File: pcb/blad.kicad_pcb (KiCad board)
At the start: 2 copper layers, 228.6 x 76.2 mm, 117 parts, among them J1 HRO_TYPE-C-31-M-12, J2 SWD, Q1 AO3401A, SW1 1U, SW10 1U, SW11 1U, SW12 1U, SW13 1.25U, SW14 1U, SW15 1U, SW16 1U, SW17 1U, SW18 1U, SW19 1U, SW2 1U, SW20 1U, SW21 1U, SW22 1U, SW23 1.75U, SW24 1.75U, SW25 1U, SW26 1U, SW27 1U, SW28 1U, SW29 1U, SW3 1U, SW30 1U, SW31 1U, SW32 1U, SW33 1U, SW34 1.25U, SW35 1.25U, SW36 1U, SW37 1.25U, SW38 2.75U, SW39 2.25U, SW4 1U, SW40 1.25U, SW41 1U, SW42 1.25U, SW5 1U, SW6 1U, SW7 1U, SW8 1U, SW9 1U, U1 SRV05-4, U2 MS88SF21 1Y40AI-U

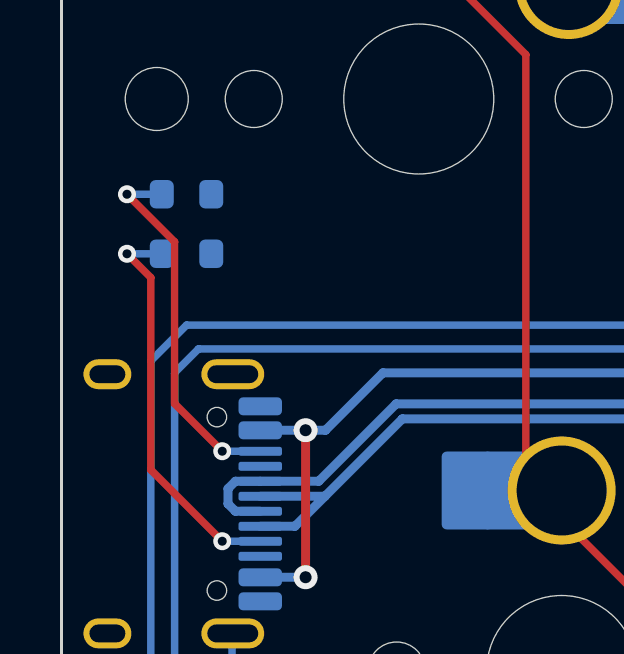
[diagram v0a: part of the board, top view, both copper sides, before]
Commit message: Refactor application implementation
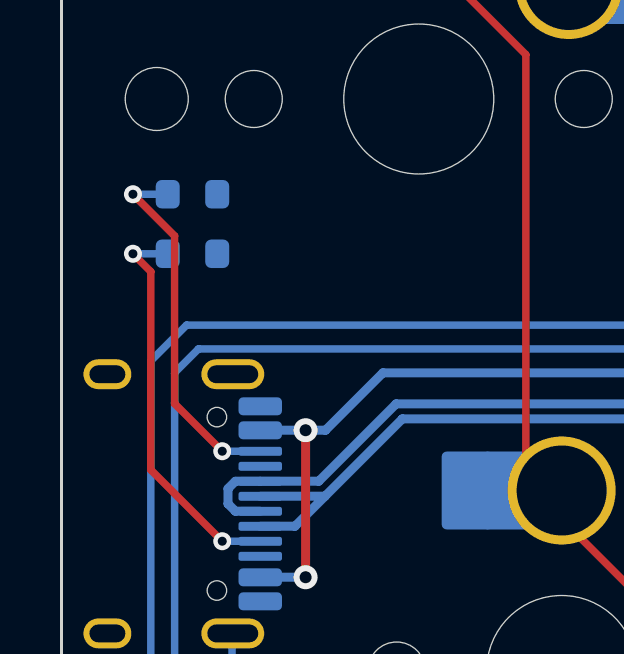
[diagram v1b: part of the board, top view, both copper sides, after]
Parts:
- moved R1 0.20 mm to (94.1, 143.3)
- moved R3 0.20 mm to (94.1, 141.3)
